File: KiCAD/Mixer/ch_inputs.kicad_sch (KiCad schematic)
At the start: 0 parts

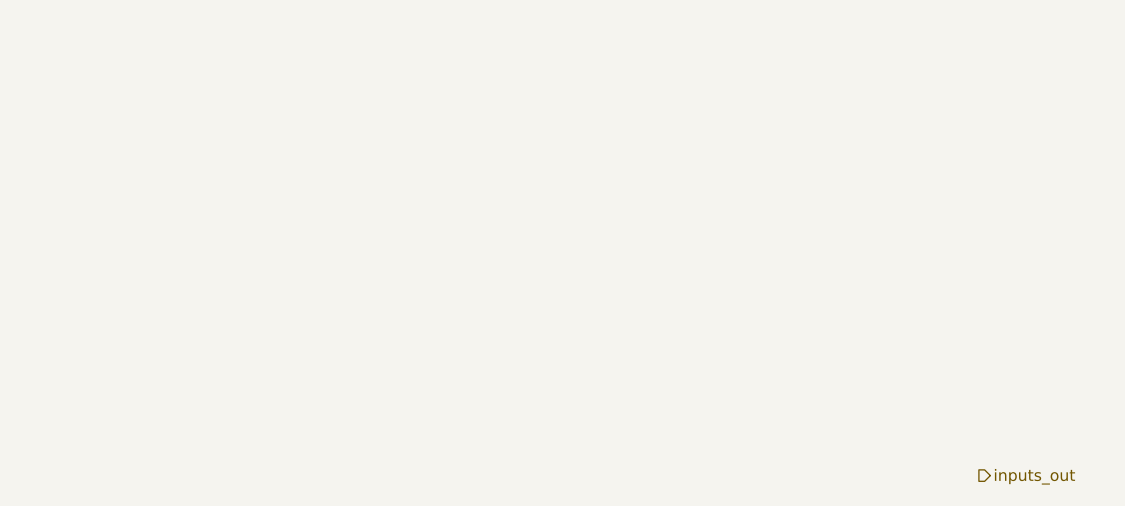
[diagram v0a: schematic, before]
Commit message: Power Bus, Footprints, Audio Bus
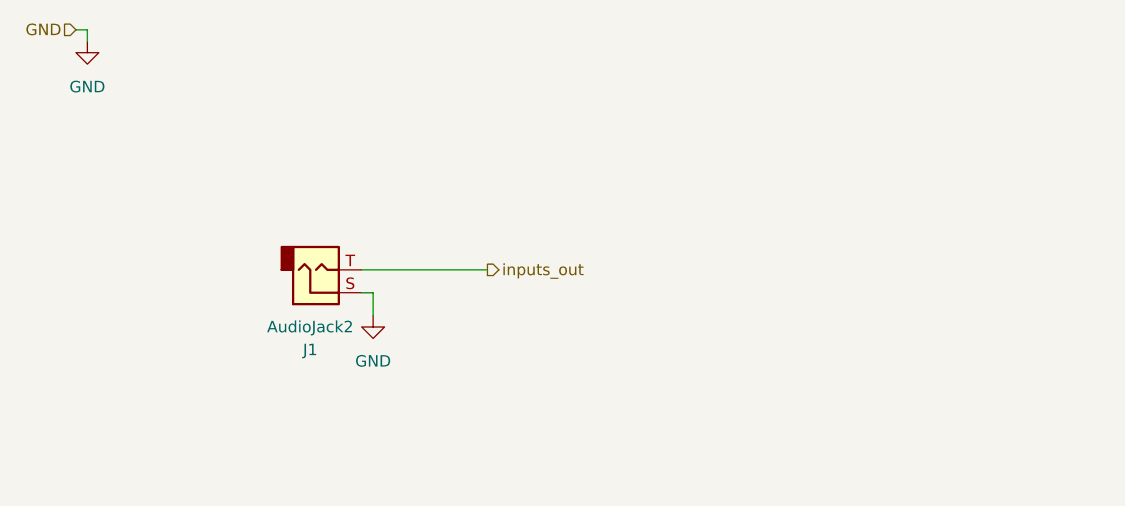
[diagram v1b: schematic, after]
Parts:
- added J1: AudioJack2, Eigene:TRS-BHT 3,5mm, symbol Connector_Audio:AudioJack2
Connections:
- net inputs_out: now also J1.T
- new net GND: J1.S
